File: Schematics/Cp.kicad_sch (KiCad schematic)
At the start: 56 parts, among them Q10 J201, Q11 J201, Q3 2SC1815, Q4 2SC1815, Q5 2SC1815, Q6 2SC1815, Q7 2SC1815, Q8 2SC1815, SW1 SW_DPDT_x2, U1 CA3080

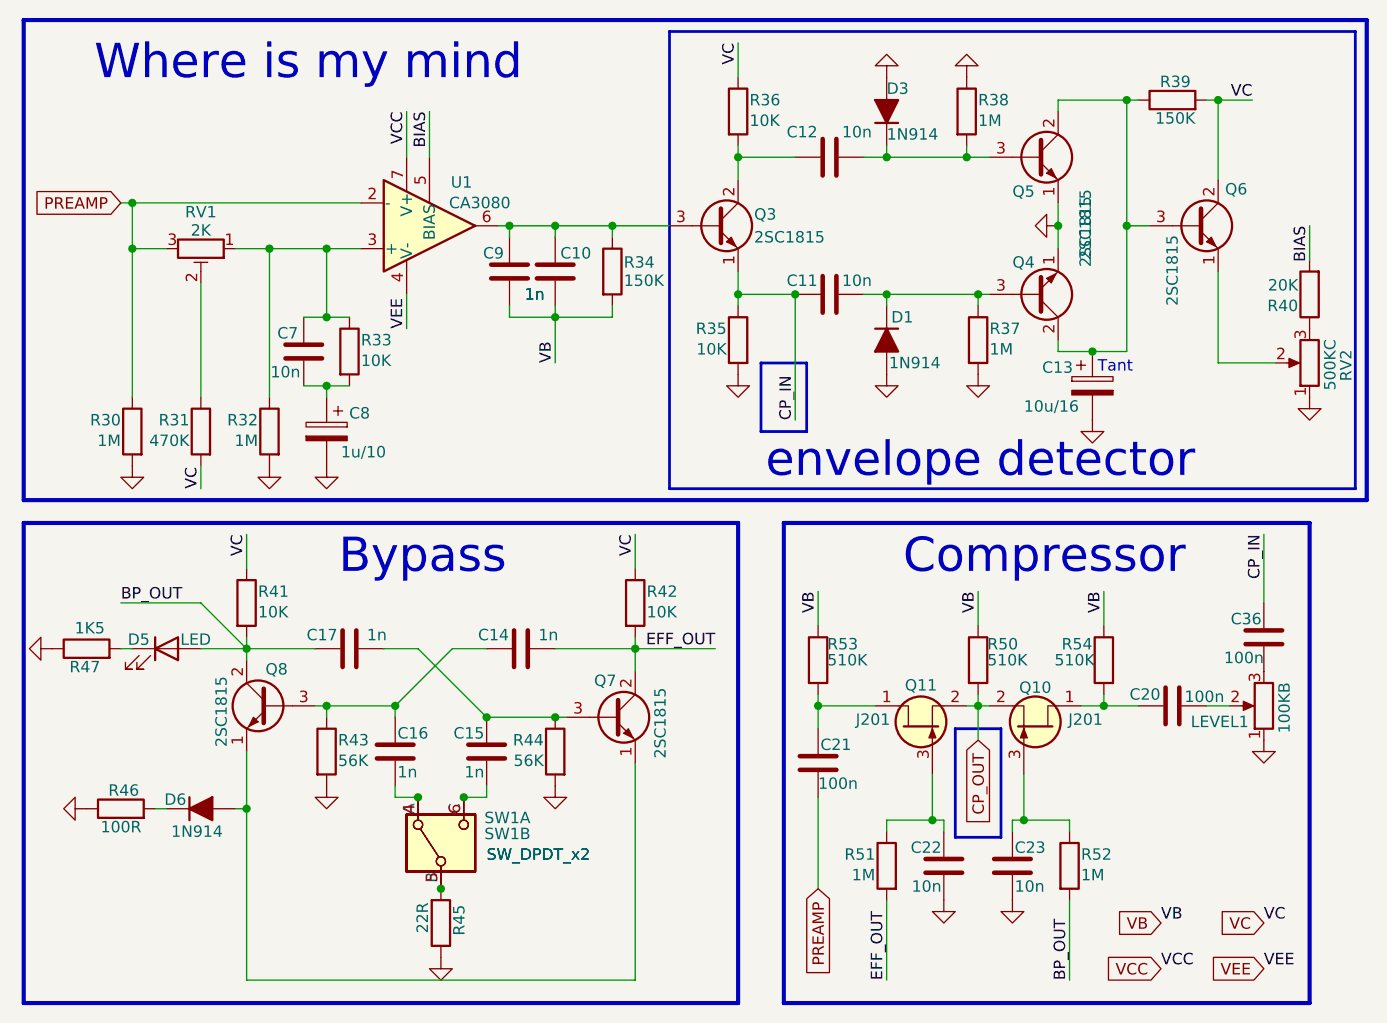
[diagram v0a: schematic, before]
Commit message: Dev(#4)
* Patch 0

PCB updates

* Patch 1

Major PCB update

* Delete AMP-MA-backups directory

* Patch 2 gitignore update

PCB update

* Repository cleaned up

* PCB upd

Traces upd, created net classes

* Beta Version 0.0.1

Traces upd, Readme Upd
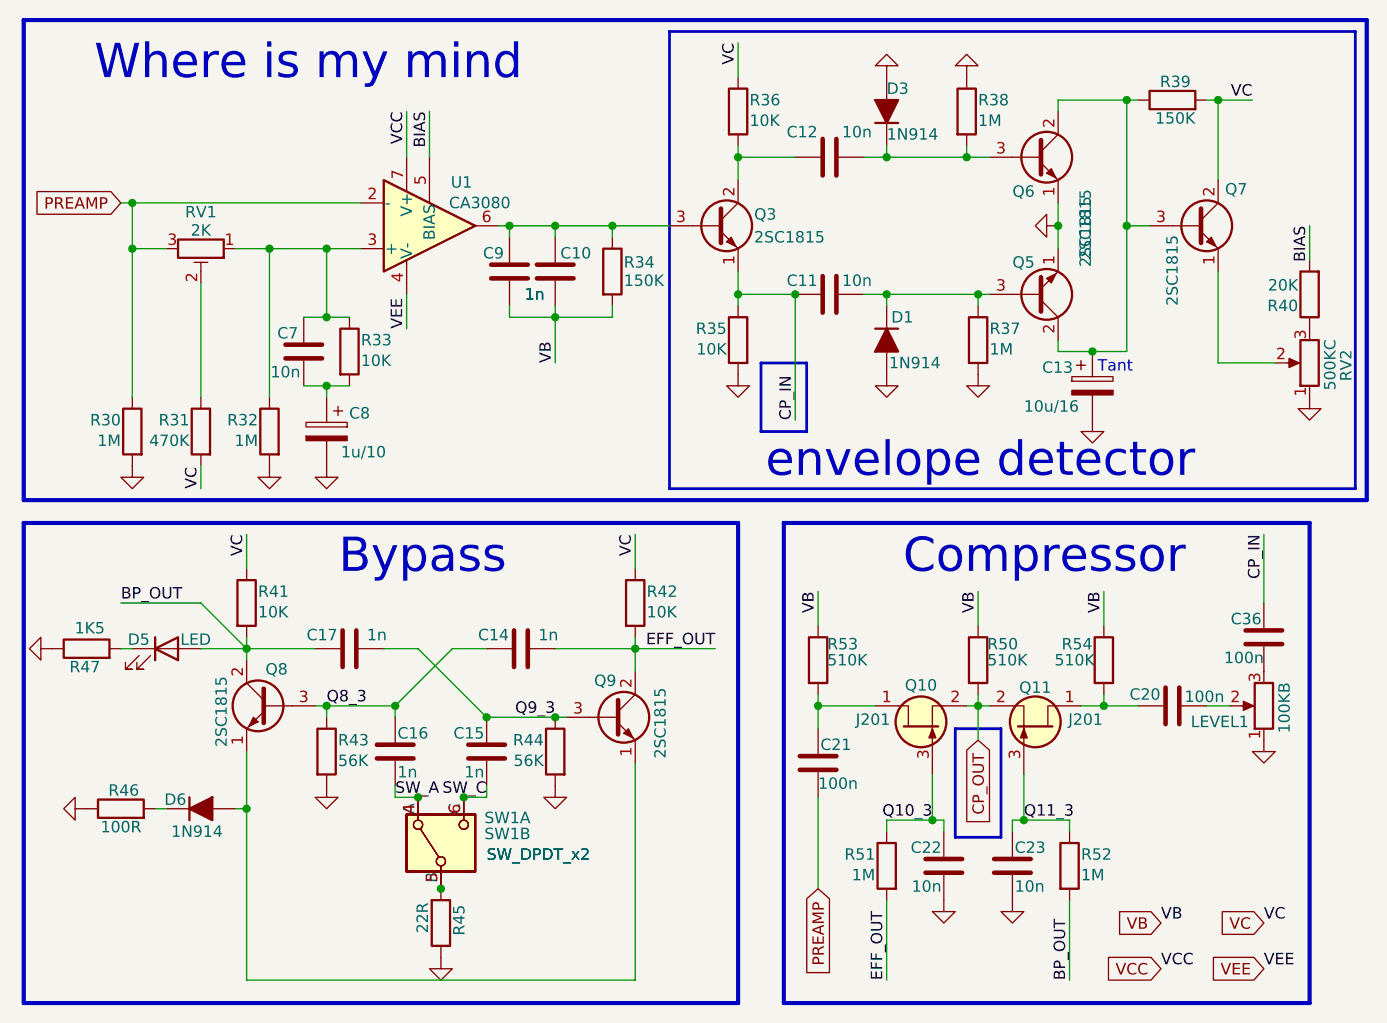
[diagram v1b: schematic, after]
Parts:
- renumbered Q11 to Q10, Q10 to Q11, Q4 to Q5, Q5 to Q6, Q6 to Q7, Q7 to Q9
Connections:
- net SW_A: now reaches C16.1, SW1.1 (A), SW1.4 (A)
- net SW_C: now reaches C15.1, SW1.3 (C), SW1.6 (C)
- net Q9_3: now reaches C15.2, C17.2, Q9.3 (B), R44.1
- net Q8_3: now reaches C14.1, C16.2, Q8.3 (B), R43.1
- net Q10_3: now reaches C22.2, Q10.3 (G), R51.1
- net Q11_3: now reaches C23.2, Q11.3 (G), R52.1
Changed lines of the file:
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@@
 	(wire
 		(pts
-			(xy 58.42 101.6) (xy 60.96 101.6)
-		)
-		(stroke
-			(width 0)
-			(type default)
-		)
-	)
-	(wire
-		(pts
 			(xy 71.12 39.37) (xy 71.12 38.1)
 		)
@@
 	(wire
 		(pts
+			(xy 58.42 101.6) (xy 60.96 101.6)
+		)
+		(stroke
+			(width 0)
+			(type default)
+		)
+	)
+	(wire
+		(pts
 			(xy 82.55 46.99) (xy 82.55 48.26)
 		)
@@
 	(wire
 		(pts
-			(xy 68.58 100.33) (xy 68.58 101.6)
-		)
-		(stroke
-			(width 0)
-			(type default)
-		)
-	)
-	(wire
-		(pts
 			(xy 27.94 80.01) (xy 36.83 80.01)
 		)
@@
 	(wire
 		(pts
-			(xy 58.42 101.6) (xy 58.42 100.33)
-		)
-		(stroke
-			(width 0)
-			(type default)
-		)
-	)
-	(wire
-		(pts
 			(xy 110.49 30.48) (xy 113.03 30.48)
 		)
@@
 	(wire
 		(pts
+			(xy 68.58 101.6) (xy 68.58 100.33)
+		)
+		(stroke
+			(width 0)
+			(type default)
+		)
+	)
+	(wire
+		(pts
 			(xy 132.08 24.13) (xy 139.7 24.13)
 		)
@@
 	(wire
 		(pts
+			(xy 58.42 101.6) (xy 58.42 100.33)
+		)
+		(stroke
+			(width 0)
+			(type default)
+		)
+	)
+	(wire
+		(pts
 			(xy 41.91 83.82) (xy 41.91 85.09)
 		)
@@
 		)
 	)
+	(label "Q10_3"
+		(at 118.11 104.14 180)
+		(effects
+			(font
+				(size 1.27 1.27)
+			)
+			(justify right bottom)
+		)
+	)
 	(label "BIAS"
 		(at 160.02 38.1 270)
@@
 		)
 	)
+	(label "SW_C"
+		(at 68.58 101.6 180)
+		(effects
+			(font
+				(size 1.27 1.27)
+			)
+			(justify right bottom)
+		)
+	)
+	(label "Q9_3"
+		(at 76.2 92.71 180)
+		(effects
+			(font
+				(size 1.27 1.27)
+			)
+			(justify right bottom)
+		)
+	)
 	(label "VC"
 		(at 96.52 17.78 270)
@@
 		)
 	)
+	(label "Q8_3"
+		(at 50.8 91.44 0)
+		(effects
+			(font
+				(size 1.27 1.27)
+			)
+			(justify left bottom)
+		)
+	)
 	(label "BP_OUT"
 		(at 133.35 121.92 90)
@@
 		)
 	)
+	(label "Q11_3"
+		(at 128.27 104.14 0)
+		(effects
+			(font
+				(size 1.27 1.27)
+			)
+			(justify left bottom)
+		)
+	)
+	(label "SW_A"
+		(at 58.42 101.6 0)
+		(effects
+			(font
+				(size 1.27 1.27)
+			)
+			(justify left bottom)
+		)
+	)
 	(global_label "VC"
 		(shape input)
@@
 		(in_pos_files yes)
 		(dnp no)
-		(property "Reference" "Q5"
+		(property "Reference" "Q6"
 			(at 127 34.29 0)
 			(show_name no)
@@
 			(project "AMP-MA"
 				(path "/4094031b-a9da-4ac5-aaa1-42b342c92a3e/d432553b-ab0c-45ec-bbdd-5af2e9267855"
-					(reference "Q5")
+					(reference "Q6")
 					(unit 1)
 				)
@@
 		(in_pos_files yes)
 		(dnp no)
-		(property "Reference" "Q11"
+		(property "Reference" "Q10"
 			(at 116.84 89.154 90)
 			(show_name no)
@@
 			(project "AMP-MA"
 				(path "/4094031b-a9da-4ac5-aaa1-42b342c92a3e/d432553b-ab0c-45ec-bbdd-5af2e9267855"
-					(reference "Q11")
+					(reference "Q10")
 					(unit 1)
 				)
@@
 		(in_pos_files yes)
 		(dnp no)
-		(property "Reference" "Q6"
+		(property "Reference" "Q7"
 			(at 150.622 34.036 0)
 			(show_name no)
@@
 			(project "AMP-MA"
 				(path "/4094031b-a9da-4ac5-aaa1-42b342c92a3e/d432553b-ab0c-45ec-bbdd-5af2e9267855"
-					(reference "Q6")
+					(reference "Q7")
 					(unit 1)
 				)
@@
 		(in_pos_files yes)
 		(dnp no)
-		(property "Reference" "Q10"
+		(property "Reference" "Q11"
 			(at 129.54 89.408 90)
 			(show_name no)
@@
 			(project "AMP-MA"
 				(path "/4094031b-a9da-4ac5-aaa1-42b342c92a3e/d432553b-ab0c-45ec-bbdd-5af2e9267855"
-					(reference "Q10")
+					(reference "Q11")
 					(unit 1)
 				)
@@
 		(in_pos_files yes)
 		(dnp no)
-		(property "Reference" "Q7"
+		(property "Reference" "Q9"
 			(at 80.518 88.646 0)
 			(show_name no)
@@
 			(project "AMP-MA"
 				(path "/4094031b-a9da-4ac5-aaa1-42b342c92a3e/d432553b-ab0c-45ec-bbdd-5af2e9267855"
-					(reference "Q7")
+					(reference "Q9")
 					(unit 1)
 				)
@@
 		(in_pos_files yes)
 		(dnp no)
-		(property "Reference" "Q4"
+		(property "Reference" "Q5"
 			(at 127 42.164 0)
 			(show_name no)
@@
 			(project "AMP-MA"
 				(path "/4094031b-a9da-4ac5-aaa1-42b342c92a3e/d432553b-ab0c-45ec-bbdd-5af2e9267855"
-					(reference "Q4")
+					(reference "Q5")
 					(unit 1)
 				)

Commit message: Revert "Beta 0.0.1"
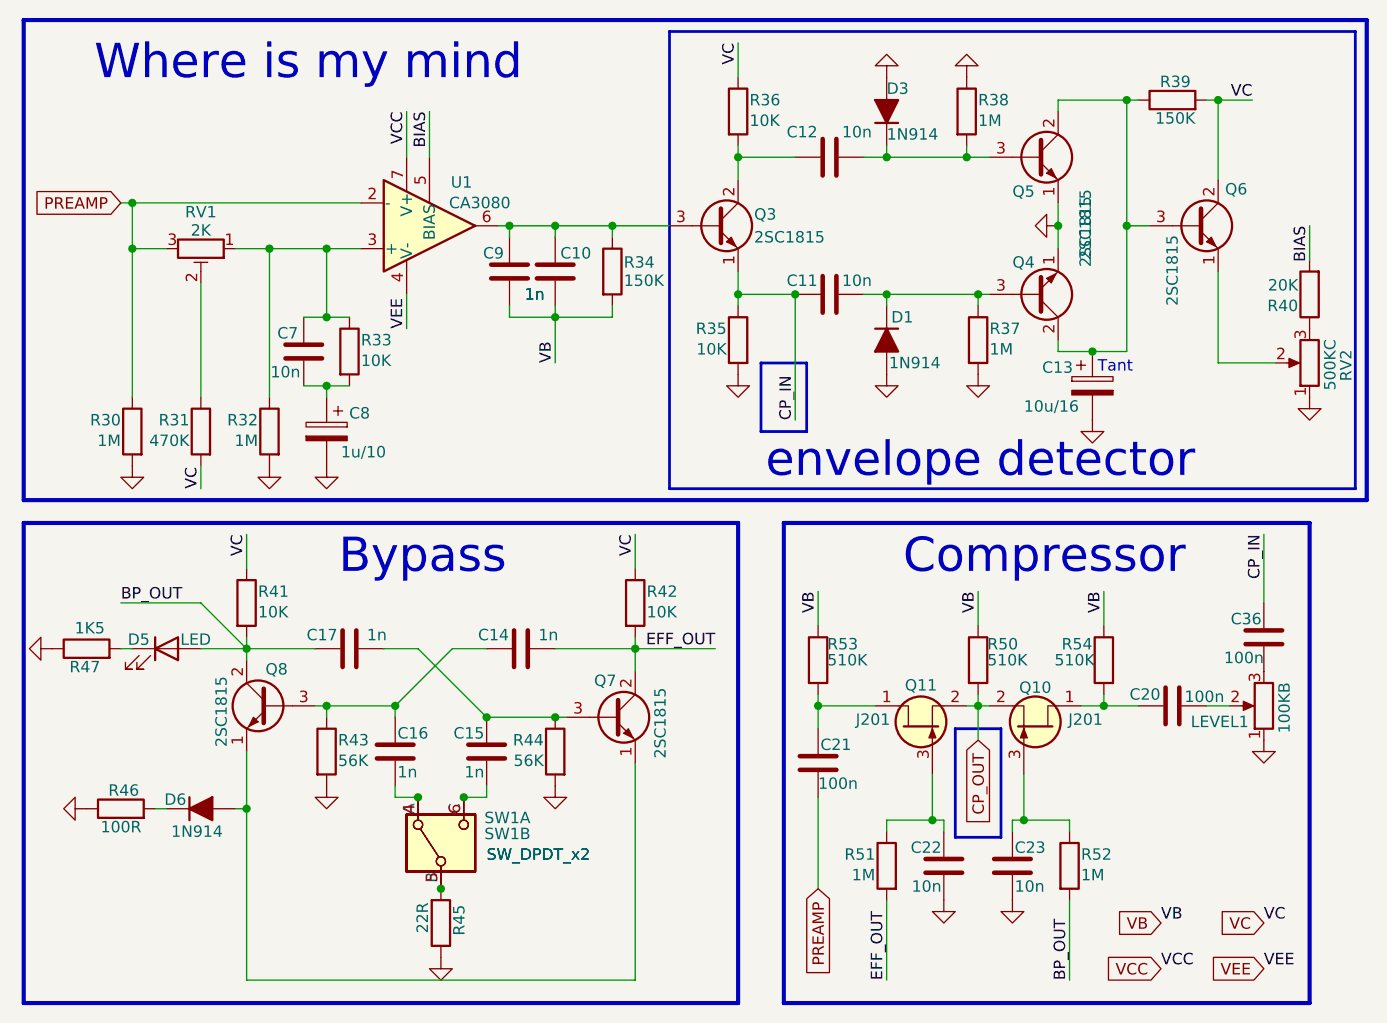
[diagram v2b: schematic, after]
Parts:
- renumbered Q11 to Q10, Q10 to Q11, Q5 to Q4, Q6 to Q5, Q7 to Q6, Q9 to Q7
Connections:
- net Q10_3: no longer names the net of C22.2, Q11.3 (G), R51.1
- net Q11_3: no longer names the net of C23.2, Q10.3 (G), R52.1
- net Q8_3: no longer names the net of C14.1, C16.2, Q8.3 (B), R43.1
- net Q9_3: no longer names the net of C15.2, C17.2, Q7.3 (B), R44.1
- net SW_A: no longer names the net of C16.1, SW1.1 (A), SW1.4 (A)
- net SW_C: no longer names the net of C15.1, SW1.3 (C), SW1.6 (C)
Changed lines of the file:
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@@
 	(wire
 		(pts
+			(xy 58.42 101.6) (xy 60.96 101.6)
+		)
+		(stroke
+			(width 0)
+			(type default)
+		)
+	)
+	(wire
+		(pts
 			(xy 71.12 39.37) (xy 71.12 38.1)
 		)
@@
 	(wire
 		(pts
-			(xy 58.42 101.6) (xy 60.96 101.6)
-		)
-		(stroke
-			(width 0)
-			(type default)
-		)
-	)
-	(wire
-		(pts
 			(xy 82.55 46.99) (xy 82.55 48.26)
 		)
@@
 	(wire
 		(pts
+			(xy 68.58 100.33) (xy 68.58 101.6)
+		)
+		(stroke
+			(width 0)
+			(type default)
+		)
+	)
+	(wire
+		(pts
 			(xy 27.94 80.01) (xy 36.83 80.01)
 		)
@@
 	(wire
 		(pts
-			(xy 110.49 30.48) (xy 113.03 30.48)
+			(xy 58.42 101.6) (xy 58.42 100.33)
 		)
 		(stroke
@@
 	(wire
 		(pts
-			(xy 124.46 45.72) (xy 123.19 45.72)
+			(xy 110.49 30.48) (xy 113.03 30.48)
 		)
 		(stroke
@@
 	(wire
 		(pts
-			(xy 27.94 35.56) (xy 29.21 35.56)
+			(xy 124.46 45.72) (xy 123.19 45.72)
 		)
 		(stroke
@@
 	(wire
 		(pts
-			(xy 68.58 92.71) (xy 76.2 92.71)
+			(xy 27.94 35.56) (xy 29.21 35.56)
 		)
 		(stroke
@@
 	(wire
 		(pts
-			(xy 123.19 82.55) (xy 123.19 78.74)
+			(xy 68.58 92.71) (xy 76.2 92.71)
 		)
 		(stroke
@@
 	(wire
 		(pts
-			(xy 132.08 52.07) (xy 132.08 50.8)
+			(xy 123.19 82.55) (xy 123.19 78.74)
 		)
 		(stroke
@@
 	(wire
 		(pts
-			(xy 76.2 48.26) (xy 76.2 46.99)
+			(xy 132.08 52.07) (xy 132.08 50.8)
 		)
 		(stroke
@@
 	(wire
 		(pts
-			(xy 142.24 38.1) (xy 139.7 38.1)
+			(xy 76.2 48.26) (xy 76.2 46.99)
 		)
 		(stroke
@@
 	(wire
 		(pts
-			(xy 68.58 101.6) (xy 68.58 100.33)
+			(xy 142.24 38.1) (xy 139.7 38.1)
 		)
 		(stroke
@@
 	(wire
 		(pts
-			(xy 58.42 101.6) (xy 58.42 100.33)
-		)
-		(stroke
-			(width 0)
-			(type default)
-		)
-	)
-	(wire
-		(pts
 			(xy 41.91 83.82) (xy 41.91 85.09)
 		)
@@
 		)
 	)
-	(label "Q10_3"
-		(at 118.11 104.14 180)
-		(effects
-			(font
-				(size 1.27 1.27)
-			)
-			(justify right bottom)
-		)
-	)
 	(label "BIAS"
 		(at 160.02 38.1 270)
@@
 		)
 	)
-	(label "SW_C"
-		(at 68.58 101.6 180)
-		(effects
-			(font
-				(size 1.27 1.27)
-			)
-			(justify right bottom)
-		)
-	)
-	(label "Q9_3"
-		(at 76.2 92.71 180)
-		(effects
-			(font
-				(size 1.27 1.27)
-			)
-			(justify right bottom)
-		)
-	)
 	(label "VC"
 		(at 96.52 17.78 270)
@@
 		)
 	)
-	(label "Q8_3"
-		(at 50.8 91.44 0)
-		(effects
-			(font
-				(size 1.27 1.27)
-			)
-			(justify left bottom)
-		)
-	)
 	(label "BP_OUT"
 		(at 133.35 121.92 90)
@@
 		)
 	)
-	(label "Q11_3"
-		(at 128.27 104.14 0)
-		(effects
-			(font
-				(size 1.27 1.27)
-			)
-			(justify left bottom)
-		)
-	)
-	(label "SW_A"
-		(at 58.42 101.6 0)
-		(effects
-			(font
-				(size 1.27 1.27)
-			)
-			(justify left bottom)
-		)
-	)
 	(global_label "VC"
 		(shape input)
@@
 		(in_pos_files yes)
 		(dnp no)
-		(property "Reference" "Q6"
+		(property "Reference" "Q5"
 			(at 127 34.29 0)
 			(show_name no)
@@
 			(project "AMP-MA"
 				(path "/4094031b-a9da-4ac5-aaa1-42b342c92a3e/d432553b-ab0c-45ec-bbdd-5af2e9267855"
-					(reference "Q6")
+					(reference "Q5")
 					(unit 1)
 				)
@@
 		(in_pos_files yes)
 		(dnp no)
-		(property "Reference" "Q10"
+		(property "Reference" "Q11"
 			(at 116.84 89.154 90)
 			(show_name no)
@@
 			(project "AMP-MA"
 				(path "/4094031b-a9da-4ac5-aaa1-42b342c92a3e/d432553b-ab0c-45ec-bbdd-5af2e9267855"
-					(reference "Q10")
+					(reference "Q11")
 					(unit 1)
 				)
@@
 		(in_pos_files yes)
 		(dnp no)
-		(property "Reference" "Q7"
+		(property "Reference" "Q6"
 			(at 150.622 34.036 0)
 			(show_name no)
@@
 			(project "AMP-MA"
 				(path "/4094031b-a9da-4ac5-aaa1-42b342c92a3e/d432553b-ab0c-45ec-bbdd-5af2e9267855"
-					(reference "Q7")
+					(reference "Q6")
 					(unit 1)
 				)
@@
 		(in_pos_files yes)
 		(dnp no)
-		(property "Reference" "Q11"
+		(property "Reference" "Q10"
 			(at 129.54 89.408 90)
 			(show_name no)
@@
 			(project "AMP-MA"
 				(path "/4094031b-a9da-4ac5-aaa1-42b342c92a3e/d432553b-ab0c-45ec-bbdd-5af2e9267855"
-					(reference "Q11")
+					(reference "Q10")
 					(unit 1)
 				)
@@
 		(in_pos_files yes)
 		(dnp no)
-		(property "Reference" "Q9"
+		(property "Reference" "Q7"
 			(at 80.518 88.646 0)
 			(show_name no)
@@
 			(project "AMP-MA"
 				(path "/4094031b-a9da-4ac5-aaa1-42b342c92a3e/d432553b-ab0c-45ec-bbdd-5af2e9267855"
-					(reference "Q9")
+					(reference "Q7")
 					(unit 1)
 				)
@@
 		(in_pos_files yes)
 		(dnp no)
-		(property "Reference" "Q5"
+		(property "Reference" "Q4"
 			(at 127 42.164 0)
 			(show_name no)
@@
 			(project "AMP-MA"
 				(path "/4094031b-a9da-4ac5-aaa1-42b342c92a3e/d432553b-ab0c-45ec-bbdd-5af2e9267855"
-					(reference "Q5")
+					(reference "Q4")
 					(unit 1)
 				)
